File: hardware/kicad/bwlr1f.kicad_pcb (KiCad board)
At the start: 4 copper layers, 64.7 x 26.1 mm, 70 parts, among them J1 Conn_01x02, Q1 PMV32UP, Q2 PMV32UP, Q3 DMG1012UW, U1 RAK3172-SIP, U2 NBM7100ABQX, U3 ZD24C08A, U4 BME688, U5 TPL5110

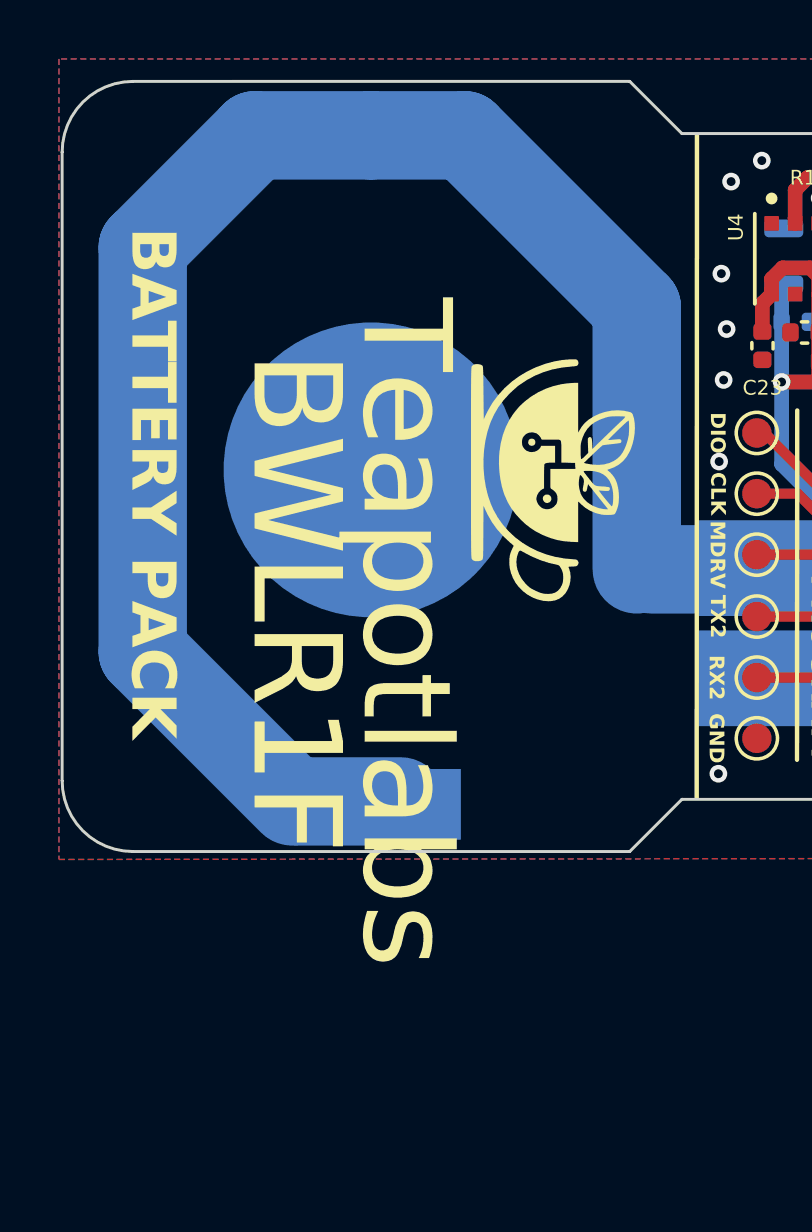
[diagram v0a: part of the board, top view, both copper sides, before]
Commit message: Revert "update layout"
This reverts commit 7d4c2235c3ae4d9f911583b993bcb32887b0ae1e.
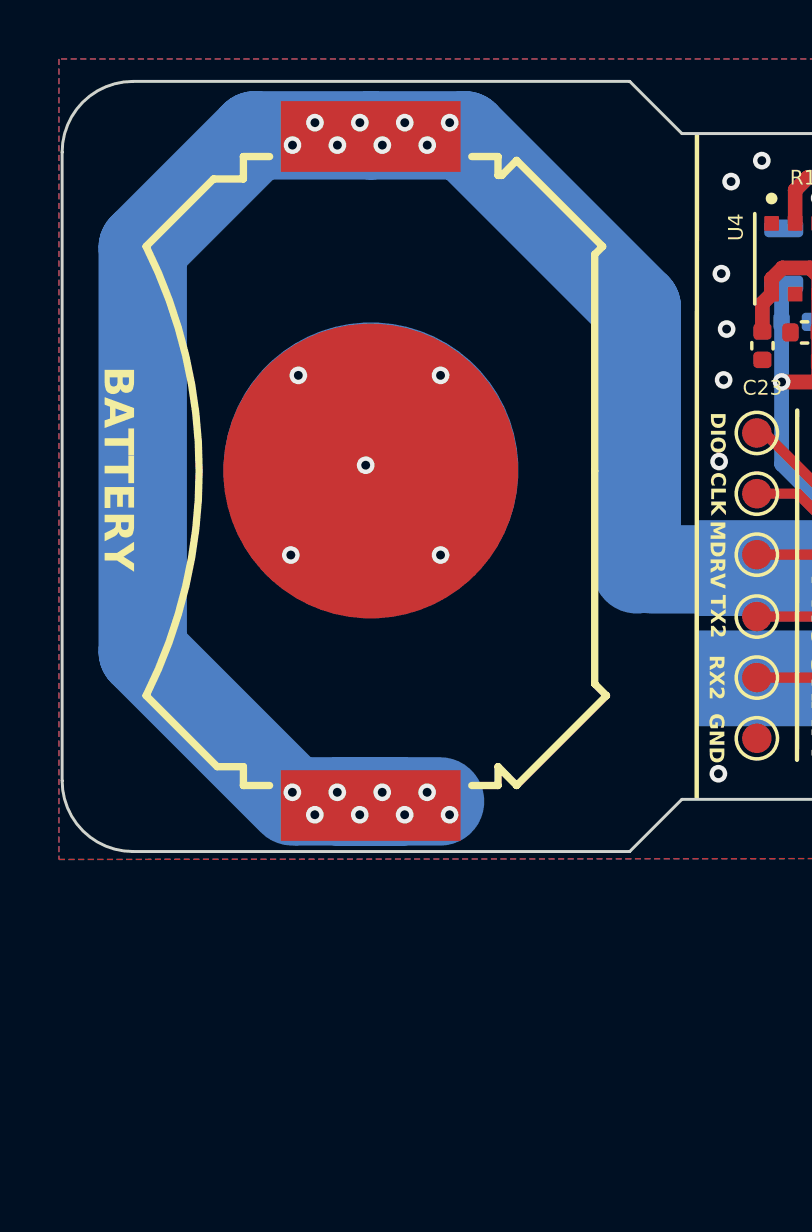
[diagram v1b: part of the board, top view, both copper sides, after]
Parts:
- removed the G*** at (122.2, 110.6)
- added BT2: Battery_Cell, bwlr1f:BAT-SMD_MY-2032-12, F.Cu at (115.9, 110.7)
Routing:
- net /BATT+: track 103.8 -> 107.2 mm, vias 5 -> 21
- net GND: vias 72 -> 77
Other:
- board text removed: "BATTERY PACK"

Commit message: update layout
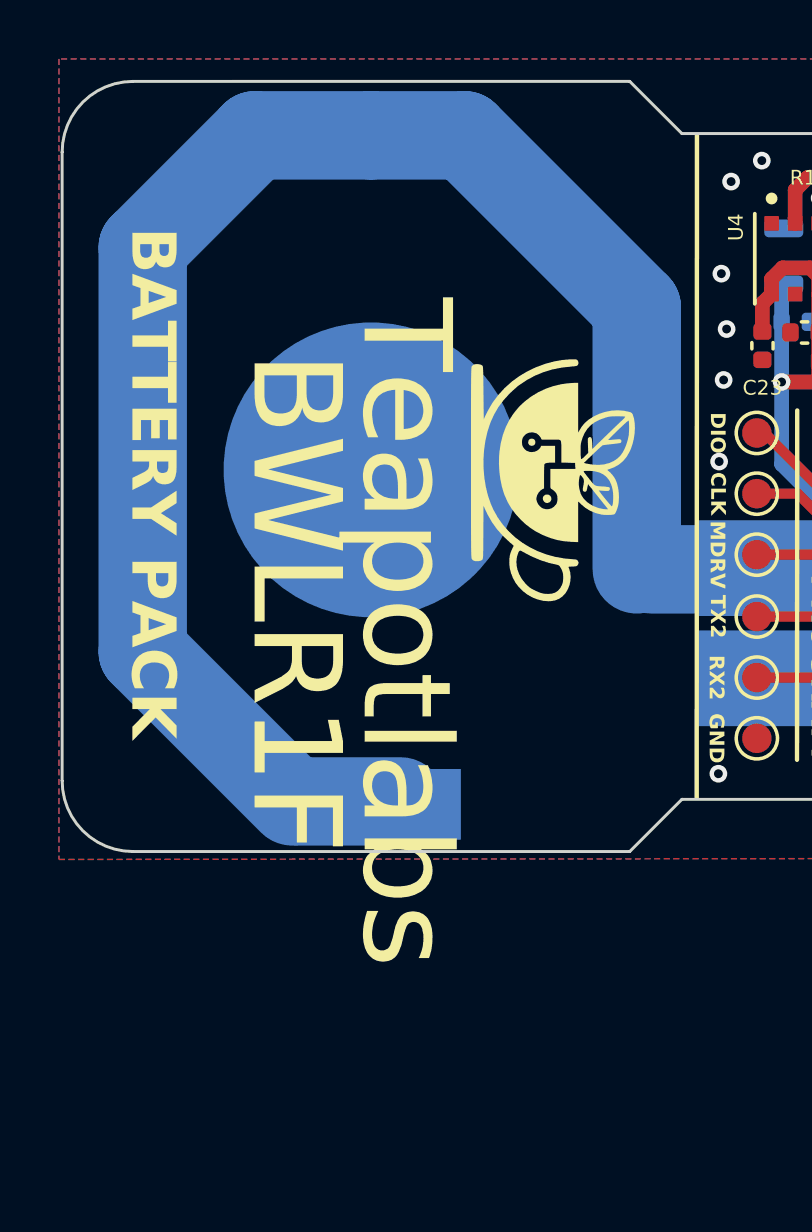
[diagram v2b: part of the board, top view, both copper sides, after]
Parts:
- removed BT2: Battery_Cell, bwlr1f:BAT-SMD_MY-2032-12
- added G***: LOGO, bwlr1f:TeapotLogo, F.Cu at (122.2, 110.6)
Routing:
- net /BATT+: track 107.2 -> 103.8 mm, vias 21 -> 5
- net GND: vias 77 -> 72
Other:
- board text added: "BATTERY PACK"
